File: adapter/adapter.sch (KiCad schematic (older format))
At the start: 6 parts, among them J1 Conn_01x04_Male, J2 RJ45, J3 Conn_01x02_Male

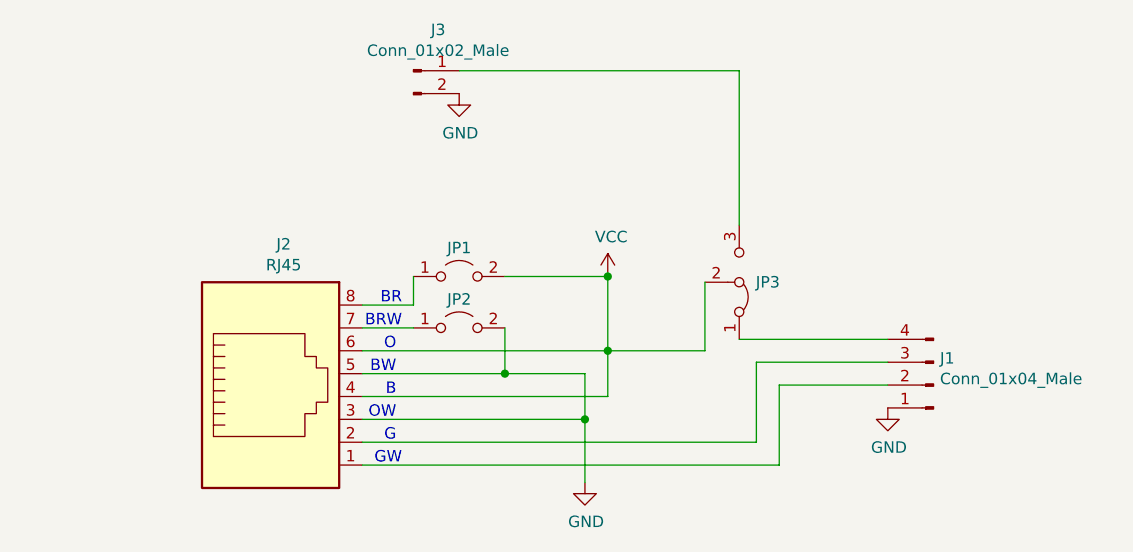
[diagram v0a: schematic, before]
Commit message: Add some adapter and interconnect pics
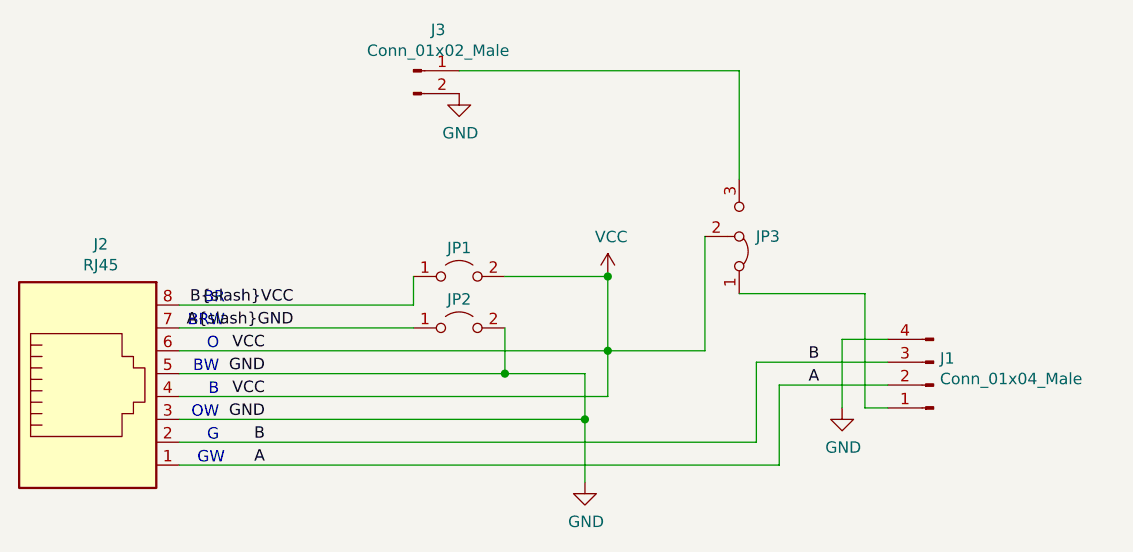
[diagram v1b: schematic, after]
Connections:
- net GND: now also J1.4 (Pin_4); no longer J1.1 (Pin_1)
- net A: now reaches J1.2 (Pin_2), J2.1
- net B: now reaches J1.3 (Pin_3), J2.2
- net A/GND: now reaches J2.7, JP2.1 (A)
- net B/VCC: now reaches J2.8, JP1.1 (A)
- net at JP3.1 (A): now also J1.1 (Pin_1); no longer J1.4 (Pin_4)
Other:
- moved on the sheet: J2, JP3
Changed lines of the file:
@@
 Comment9 ""
 $EndDescr
-Wire Wire Line
-	3550 4700 5275 4700
-Wire Wire Line
-	4625 4300 3550 4300
-Wire Wire Line
-	4525 4600 3550 4600
-Wire Wire Line
-	4625 4500 3550 4500
+Connection ~ 4175 4400
+Connection ~ 4525 4600
+Connection ~ 4625 3975
+Connection ~ 4625 4300
+Wire Wire Line
+	2750 4100 3775 4100
+Wire Wire Line
+	2750 4200 3775 4200
+Wire Wire Line
+	2750 4700 5275 4700
+Wire Wire Line
+	2750 4800 5375 4800
+Wire Wire Line
+	3775 4100 3775 3975
+Wire Wire Line
+	3975 3075 5200 3075
+Wire Wire Line
+	4175 3975 4625 3975
+Wire Wire Line
+	4175 4200 4175 4400
+Wire Wire Line
+	4175 4400 2750 4400
 Wire Wire Line
 	4525 4400 4175 4400
 Wire Wire Line
-	5200 4250 5850 4250
+	4525 4400 4525 4600
+Wire Wire Line
+	4525 4600 2750 4600
+Wire Wire Line
+	4525 4600 4525 4875
+Wire Wire Line
+	4625 3975 4625 4300
+Wire Wire Line
+	4625 4300 2750 4300
+Wire Wire Line
+	4625 4300 4625 4500
+Wire Wire Line
+	4625 4300 5050 4300
+Wire Wire Line
+	4625 4500 2750 4500
+Wire Wire Line
+	5050 4300 5050 3800
+Wire Wire Line
+	5200 3075 5200 3550
+Wire Wire Line
+	5200 4050 5750 4050
+Wire Wire Line
+	5275 4350 5850 4350
+Wire Wire Line
+	5275 4700 5275 4350
+Wire Wire Line
+	5375 4450 5850 4450
 Wire Wire Line
 	5375 4800 5375 4450
 Wire Wire Line
-	5375 4450 5850 4450
-Wire Wire Line
-	5275 4350 5850 4350
-Wire Wire Line
-	5275 4700 5275 4350
+	5650 4250 5650 4550
+Wire Wire Line
+	5750 4050 5750 4550
+Wire Wire Line
+	5750 4550 5850 4550
+Wire Wire Line
+	5850 4250 5650 4250
+Text Notes 2925 4300 2    50   ~ 0
+O
+Text Notes 2925 4400 2    50   ~ 0
+BW
+Text Notes 2925 4500 2    50   ~ 0
+B
+Text Notes 2925 4600 2    50   ~ 0
+OW
+Text Notes 2925 4700 2    50   ~ 0
+G
+Text Notes 2950 4100 2    50   ~ 0
+BR
+Text Notes 2950 4200 2    50   ~ 0
+BRW
+Text Notes 2950 4800 2    50   ~ 0
+GW
+Text Label 3125 4300 2    50   ~ 0
+VCC
+Text Label 3125 4400 2    50   ~ 0
+GND
+Text Label 3125 4500 2    50   ~ 0
+VCC
+Text Label 3125 4600 2    50   ~ 0
+GND
+Text Label 3125 4700 2    50   ~ 0
+B
+Text Label 3125 4800 2    50   ~ 0
+A
+Text Label 3250 4100 2    50   ~ 0
+B{slash}VCC
+Text Label 3250 4200 2    50   ~ 0
+A{slash}GND
+Text Label 5550 4350 2    50   ~ 0
+B
+Text Label 5550 4450 2    50   ~ 0
+A
+$Comp
+L power:VCC #PWR?
+U 1 1 5E309DAF
+P 4625 3975
+F 0 "#PWR?" H 4625 3825 50  0001 C CNN
+F 1 "VCC" H 4640 4148 50  0000 C CNN
+F 2 "" H 4625 3975 50  0001 C CNN
+F 3 "" H 4625 3975 50  0001 C CNN
+	1    4625 3975
+	1    0    0    -1
+$EndComp
+$Comp
+L power:GND #PWR?
+U 1 1 5E310096
+P 3975 3175
+F 0 "#PWR?" H 3975 2925 50  0001 C CNN
+F 1 "GND" H 3980 3002 50  0000 C CNN
+F 2 "" H 3975 3175 50  0001 C CNN
+F 3 "" H 3975 3175 50  0001 C CNN
+	1    3975 3175
+	1    0    0    -1
+$EndComp
+$Comp
+L power:GND #PWR?
+U 1 1 5E30A136
+P 4525 4875
+F 0 "#PWR?" H 4525 4625 50  0001 C CNN
+F 1 "GND" H 4530 4702 50  0000 C CNN
+F 2 "" H 4525 4875 50  0001 C CNN
+F 3 "" H 4525 4875 50  0001 C CNN
+	1    4525 4875
+	1    0    0    -1
+$EndComp
+$Comp
+L power:GND #PWR?
+U 1 1 5E30BC3A
+P 5650 4550
+F 0 "#PWR?" H 5650 4300 50  0001 C CNN
+F 1 "GND" H 5655 4377 50  0000 C CNN
+F 2 "" H 5650 4550 50  0001 C CNN
+F 3 "" H 5650 4550 50  0001 C CNN
+	1    5650 4550
+	1    0    0    -1
+$EndComp
+$Comp
+L Connector:Conn_01x02_Male J3
+U 1 1 5E30CE36
+P 3775 3075
+F 0 "J3" H 3883 3254 50  0000 C CNN
+F 1 "Conn_01x02_Male" H 3883 3163 50  0000 C CNN
+F 2 "TerminalBlock_RND:TerminalBlock_RND_205-00287_Pitch5.08mm" H 3775 3075 50  0001 C CNN
+F 3 "~" H 3775 3075 50  0001 C CNN
+	1    3775 3075
+	1    0    0    -1
+$EndComp
+$Comp
+L Jumper:Jumper_2_Open JP1
+U 1 1 5E3170CB
+P 3975 3975
+F 0 "JP1" H 3975 4100 50  0000 C CNN
+F 1 "Jumper_2_Open" H 3975 4118 50  0001 C CNN
+F 2 "Jumper:SolderJumper-2_P1.3mm_Open_Pad1.0x1.5mm" H 3975 3975 50  0001 C CNN
+F 3 "~" H 3975 3975 50  0001 C CNN
+	1    3975 3975
+	1    0    0    -1
+$EndComp
+$Comp
+L Jumper:Jumper_2_Open JP2
+U 1 1 5E319375
+P 3975 4200
+F 0 "JP2" H 3975 4325 50  0000 C CNN
+F 1 "Jumper_2_Open" H 3975 4343 50  0001 C CNN
+F 2 "Jumper:SolderJumper-2_P1.3mm_Open_Pad1.0x1.5mm" H 3975 4200 50  0001 C CNN
+F 3 "~" H 3975 4200 50  0001 C CNN
+	1    3975 4200
+	1    0    0    -1
+$EndComp
 $Comp
 L Connector:Conn_01x04_Male J1
@@
 $EndComp
 $Comp
-L power:GND #PWR?
-U 1 1 5E30BC3A
-P 5850 4550
-F 0 "#PWR?" H 5850 4300 50  0001 C CNN
-F 1 "GND" H 5855 4377 50  0000 C CNN
-F 2 "" H 5850 4550 50  0001 C CNN
-F 3 "" H 5850 4550 50  0001 C CNN
-	1    5850 4550
-	1    0    0    -1
-$EndComp
-Connection ~ 4525 4600
-Wire Wire Line
-	4525 4400 4525 4600
-Wire Wire Line
-	4625 4300 4625 4500
-Connection ~ 4625 4300
-Connection ~ 4625 3975
-$Comp
 L Jumper:Jumper_3_Bridged12 JP3
 U 1 1 5E312537
-P 5200 4000
-F 0 "JP3" V 5200 4125 50  0000 C CNN
-F 1 "Jumper_3_Bridged12" H 5200 4112 50  0001 C CNN
-F 2 "Jumper:SolderJumper-3_P1.3mm_Bridged12_RoundedPad1.0x1.5mm_NumberLabels" H 5200 4000 50  0001 C CNN
-F 3 "~" H 5200 4000 50  0001 C CNN
-	1    5200 4000
+P 5200 3800
+F 0 "JP3" V 5200 3925 50  0000 C CNN
+F 1 "Jumper_3_Bridged12" H 5200 3912 50  0001 C CNN
+F 2 "Jumper:SolderJumper-3_P1.3mm_Bridged12_RoundedPad1.0x1.5mm_NumberLabels" H 5200 3800 50  0001 C CNN
+F 3 "~" H 5200 3800 50  0001 C CNN
+	1    5200 3800
 	0    1    -1   0
 $EndComp
-Wire Wire Line
-	4625 3975 4625 4300
-Wire Wire Line
-	5200 3075 5200 3750
-Wire Wire Line
-	4625 4300 5050 4300
-Wire Wire Line
-	5050 4300 5050 4000
-Wire Wire Line
-	3975 3075 5200 3075
-Text Notes 3700 4700 2    50   ~ 0
-G
-Text Notes 3700 4600 2    50   ~ 0
-OW
-Text Notes 3700 4500 2    50   ~ 0
-B
-Text Notes 3700 4400 2    50   ~ 0
-BW
-Wire Wire Line
-	3550 4200 3775 4200
-Wire Wire Line
-	4175 4400 3550 4400
-Wire Wire Line
-	4175 4200 4175 4400
-Text Notes 3700 4300 2    50   ~ 0
-O
-Text Notes 3725 4200 2    50   ~ 0
-BRW
-Text Notes 3725 4100 2    50   ~ 0
-BR
-Text Notes 3725 4800 2    50   ~ 0
-GW
-Wire Wire Line
-	3550 4100 3775 4100
-Wire Wire Line
-	3775 4100 3775 3975
 $Comp
 L Connector:RJ45 J2
 U 1 1 5E263AF8
-P 3150 4500
-F 0 "J2" H 3207 5166 50  0000 C CNN
-F 1 "RJ45" H 3207 5075 50  0000 C CNN
-F 2 "Connector_RJ:RJ45_Amphenol_54602-x08_Horizontal" V 3150 4525 50  0001 C CNN
-F 3 "~" V 3150 4525 50  0001 C CNN
-	1    3150 4500
-	1    0    0    -1
-$EndComp
-Wire Wire Line
-	4175 3975 4625 3975
-$Comp
-L Connector:Conn_01x02_Male J3
-U 1 1 5E30CE36
-P 3775 3075
-F 0 "J3" H 3883 3254 50  0000 C CNN
-F 1 "Conn_01x02_Male" H 3883 3163 50  0000 C CNN
-F 2 "TerminalBlock_RND:TerminalBlock_RND_205-00287_Pitch5.08mm" H 3775 3075 50  0001 C CNN
-F 3 "~" H 3775 3075 50  0001 C CNN
-	1    3775 3075
-	1    0    0    -1
-$EndComp
-$Comp
-L Jumper:Jumper_2_Open JP1
-U 1 1 5E3170CB
-P 3975 3975
-F 0 "JP1" H 3975 4100 50  0000 C CNN
-F 1 "Jumper_2_Open" H 3975 4118 50  0001 C CNN
-F 2 "Jumper:SolderJumper-2_P1.3mm_Open_Pad1.0x1.5mm" H 3975 3975 50  0001 C CNN
-F 3 "~" H 3975 3975 50  0001 C CNN
-	1    3975 3975
-	1    0    0    -1
-$EndComp
-$Comp
-L Jumper:Jumper_2_Open JP2
-U 1 1 5E319375
-P 3975 4200
-F 0 "JP2" H 3975 4325 50  0000 C CNN
-F 1 "Jumper_2_Open" H 3975 4343 50  0001 C CNN
-F 2 "Jumper:SolderJumper-2_P1.3mm_Open_Pad1.0x1.5mm" H 3975 4200 50  0001 C CNN
-F 3 "~" H 3975 4200 50  0001 C CNN
-	1    3975 4200
-	1    0    0    -1
-$EndComp
-$Comp
-L power:GND #PWR?
-U 1 1 5E310096
-P 3975 3175
-F 0 "#PWR?" H 3975 2925 50  0001 C CNN
-F 1 "GND" H 3980 3002 50  0000 C CNN
-F 2 "" H 3975 3175 50  0001 C CNN
-F 3 "" H 3975 3175 50  0001 C CNN
-	1    3975 3175
-	1    0    0    -1
-$EndComp
-$Comp
-L power:VCC #PWR?
-U 1 1 5E309DAF
-P 4625 3975
-F 0 "#PWR?" H 4625 3825 50  0001 C CNN
-F 1 "VCC" H 4640 4148 50  0000 C CNN
-F 2 "" H 4625 3975 50  0001 C CNN
-F 3 "" H 4625 3975 50  0001 C CNN
-	1    4625 3975
-	1    0    0    -1
-$EndComp
-Connection ~ 4175 4400
-Wire Wire Line
-	3550 4800 5375 4800
-Wire Wire Line
-	4525 4600 4525 4875
-$Comp
-L power:GND #PWR?
-U 1 1 5E30A136
-P 4525 4875
-F 0 "#PWR?" H 4525 4625 50  0001 C CNN
-F 1 "GND" H 4530 4702 50  0000 C CNN
-F 2 "" H 4525 4875 50  0001 C CNN
-F 3 "" H 4525 4875 50  0001 C CNN
-	1    4525 4875
-	1    0    0    -1
-$EndComp
+P 2350 4500
+F 0 "J2" H 2407 5166 50  0000 C CNN
+F 1 "RJ45" H 2407 5075 50  0000 C CNN
+F 2 "Connector_RJ:RJ45_Amphenol_54602-x08_Horizontal" V 2350 4525 50  0001 C CNN
+F 3 "~" V 2350 4525 50  0001 C CNN
+	1    2350 4500
+	1    0    0    -1
+$EndComp
